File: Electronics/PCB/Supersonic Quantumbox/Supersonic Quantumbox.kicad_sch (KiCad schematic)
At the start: 41 parts, among them J1 USB_C_Receptacle_USB2.0, U1 Input_jack, U2 TL071, U3 PCM1808PWR, U4 AZ1117-5.0, U5 ESP32-S2-WROVER-I, U6 AZ1117-3.3, U7 PCM5100, U8 Output_jack

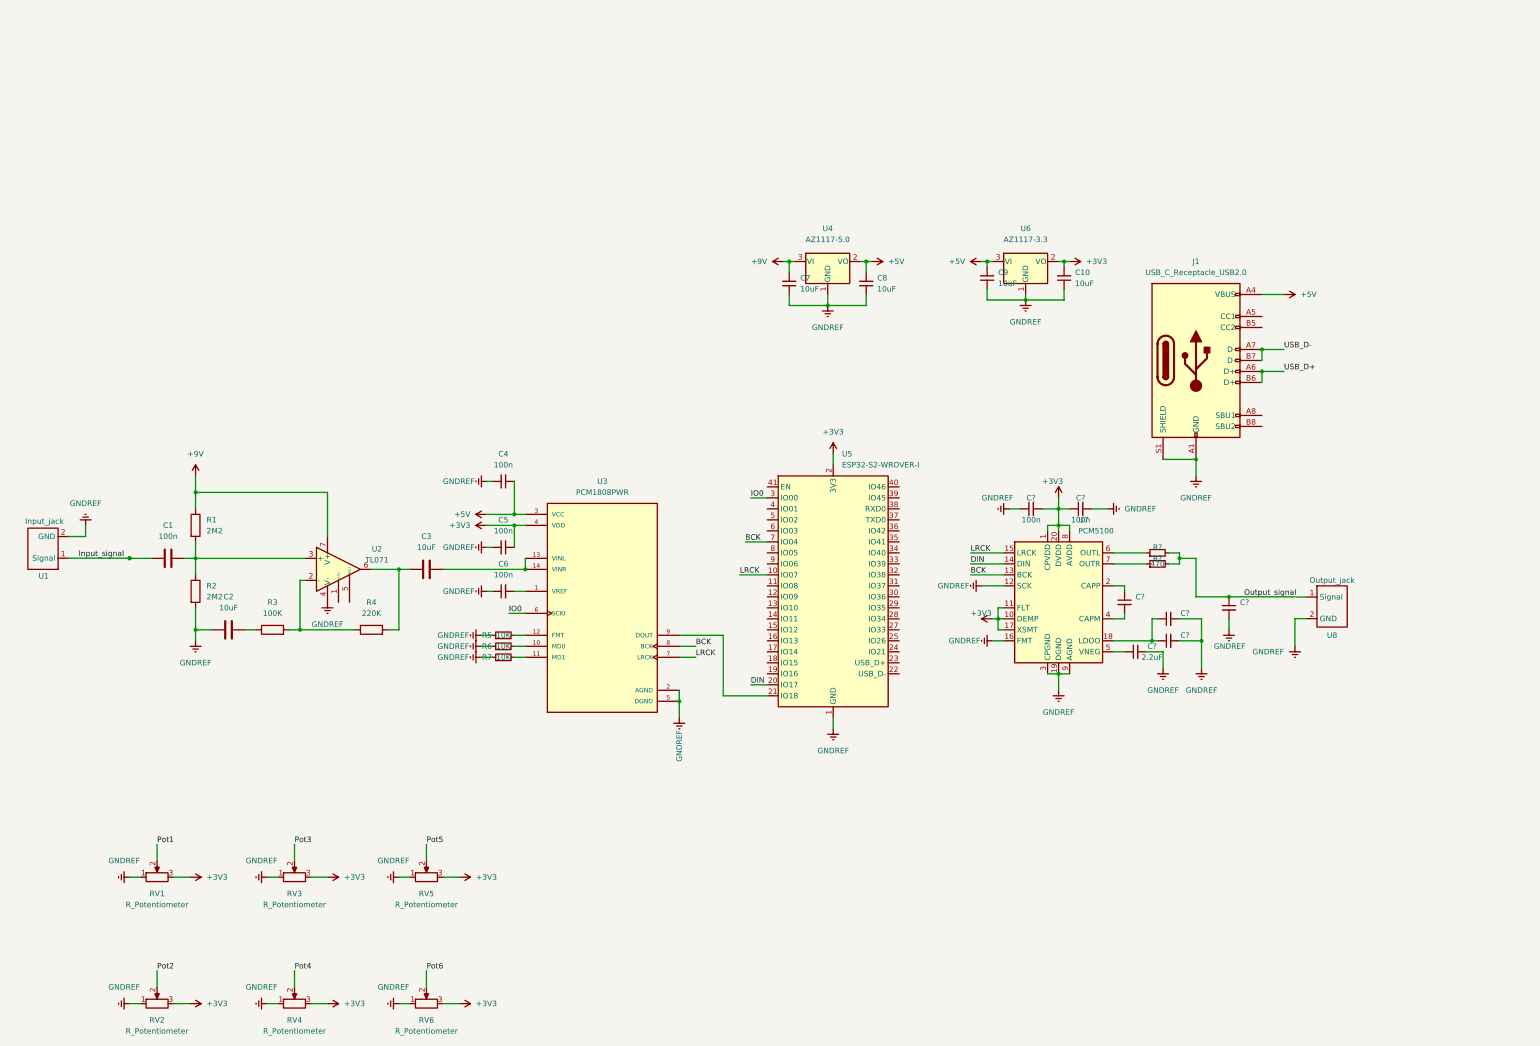
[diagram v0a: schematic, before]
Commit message: Start work on PCB
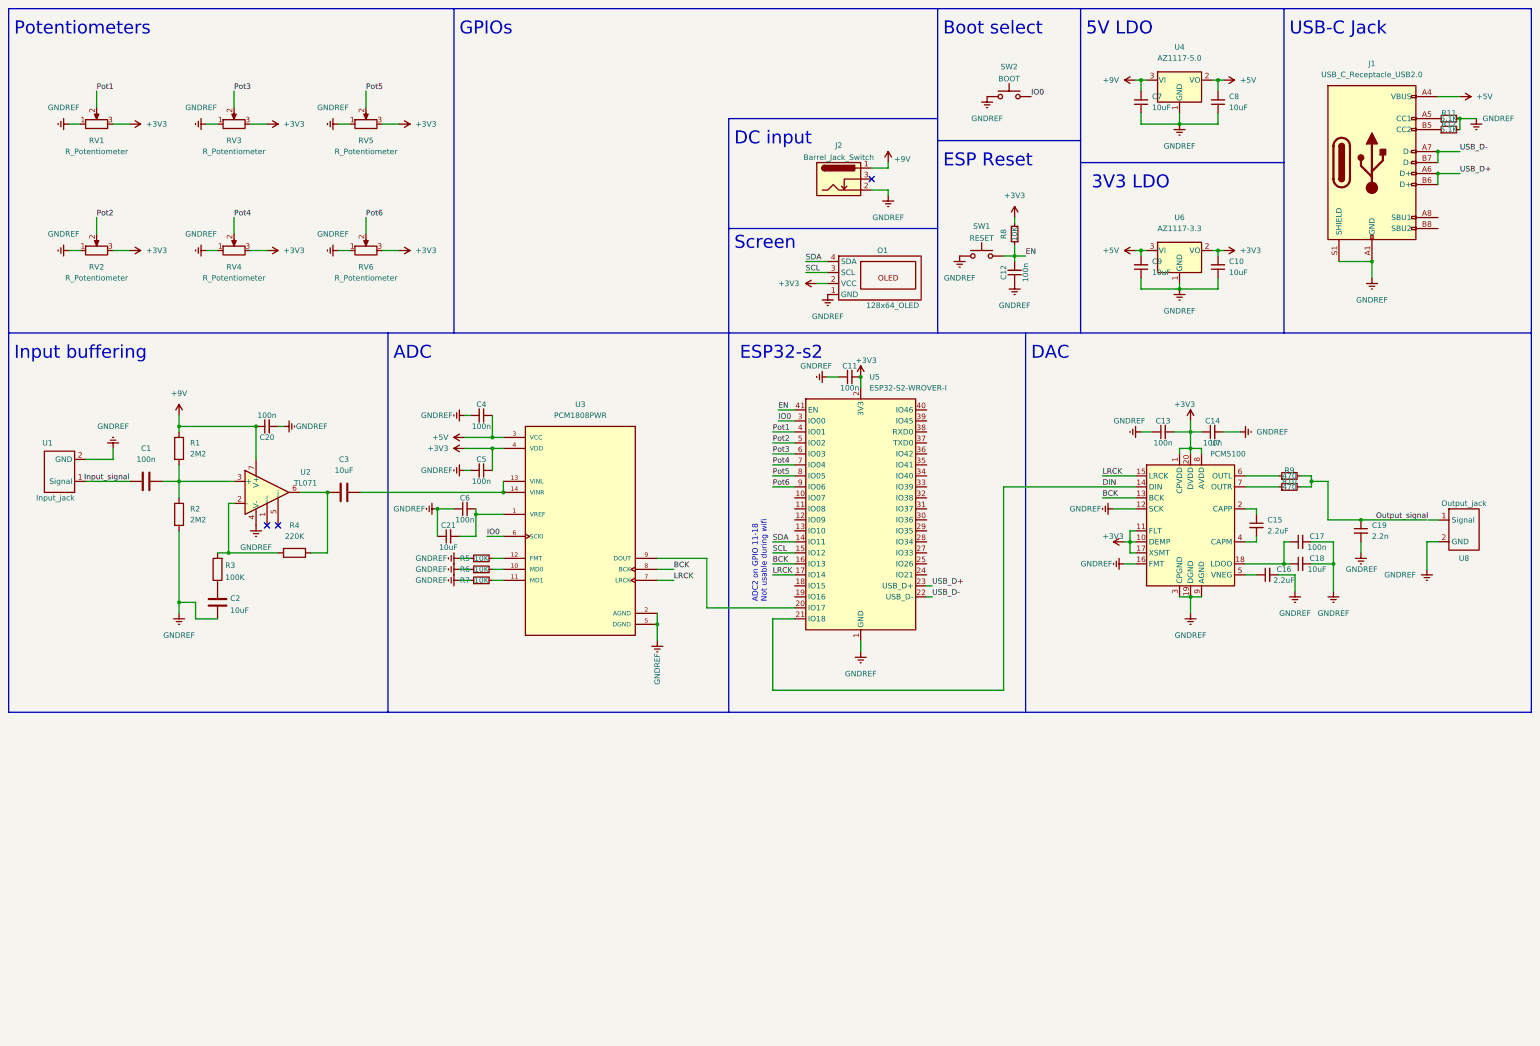
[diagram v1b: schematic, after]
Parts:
- added C11, C12, C20: 100n, Capacitor_SMD:C_0805_2012Metric_Pad1.18x1.45mm_HandSolder, symbol Device:C_Small
- added C21: 10uF, Capacitor_SMD:C_1206_3216Metric, symbol Device:C_Small
- added J2: Barrel_Jack_Switch, Connector_BarrelJack:BarrelJack_Horizontal, symbol Connector:Barrel_Jack_Switch
- added O1: 128x64_OLED, SupersonicQuantumbox:128x64OLED, symbol SupersonicQuantumbox:128x64_OLED
- added R11, R12: 5.1K, Resistor_SMD:R_0805_2012Metric_Pad1.20x1.40mm_HandSolder, symbol Device:R_Small
- added R8: 10K, Resistor_SMD:R_0805_2012Metric_Pad1.20x1.40mm_HandSolder, symbol Device:R_Small
- added SW1: RESET, Button_Switch_SMD:SW_Push_1P1T_NO_6x6mm_H9.5mm, symbol Switch:SW_Push
- added SW2: BOOT, Button_Switch_SMD:SW_Push_1P1T_NO_6x6mm_H9.5mm, symbol Switch:SW_Push
- C1, C4, C5, C6: footprint (none) -> Capacitor_SMD:C_0805_2012Metric_Pad1.18x1.45mm_HandSolder
- C10, C2, C3, C7, C8, C9: footprint (none) -> Capacitor_SMD:C_1206_3216Metric
- C13, C14: renamed from C?; footprint (none) -> Capacitor_SMD:C_0805_2012Metric_Pad1.18x1.45mm_HandSolder
- C15: renamed from C?; value (none) -> 2.2uF; footprint (none) -> Capacitor_SMD:C_1206_3216Metric
- C16: renamed from C?; footprint (none) -> Capacitor_SMD:C_1206_3216Metric
- C17: renamed from C?; value (none) -> 100n; footprint (none) -> Capacitor_SMD:C_0805_2012Metric_Pad1.18x1.45mm_HandSolder
- C18: renamed from C?; value (none) -> 10uF; footprint (none) -> Capacitor_SMD:C_1206_3216Metric
- C19: renamed from C?; value (none) -> 2.2n; footprint (none) -> Capacitor_SMD:C_0805_2012Metric_Pad1.18x1.45mm_HandSolder
- R1, R2, R3, R4, R5, R6, R7: footprint (none) -> Resistor_SMD:R_0805_2012Metric_Pad1.20x1.40mm_HandSolder
- R10: renamed from R?; footprint (none) -> Resistor_SMD:R_0805_2012Metric_Pad1.20x1.40mm_HandSolder
- R9: renamed from R?; value (none) -> 470; footprint (none) -> Resistor_SMD:R_0805_2012Metric_Pad1.20x1.40mm_HandSolder
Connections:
- net +3V3: now also C11.2, O1.2 (VCC), R8.2
- net +9V: now also C20.1, J2.1
- net BCK: now also U5.16 (IO13); no longer U5.7 (IO04)
- net DIN: now also U5.21 (IO18); no longer U5.20 (IO17)
- net GNDREF: now also C11.1, C12.1, C20.2, C21.1, J2.2, O1.1 (GND), R11.2, R12.2, SW1.1, SW2.1
- net IO0: now also SW2.2
- net LRCK: now also U5.17 (IO14); no longer U5.10 (IO07)
- net Pot1: now also U5.4 (IO01)
- net Pot2: now also U5.5 (IO02)
- net Pot3: now also U5.6 (IO03)
- net Pot4: now also U5.7 (IO04)
- net Pot5: now also U5.8 (IO05)
- net Pot6: now also U5.9 (IO06)
- net USB_D+: now also U5.23 (USB_D+)
- net USB_D-: now also U5.22 (USB_D-)
- net at C6.2, U3.1 (VREF): now also C21.2
- net at U3.9 (DOUT): now also U5.20 (IO17); no longer U5.21 (IO18)
- net SDA: now reaches U5.14 (IO11)
- net SDA: now also O1.4 (SDA)
- net SCL: now reaches U5.15 (IO12)
- net SCL: now also O1.3 (SCL)
- net EN: now reaches U5.41 (EN)
- net EN: now also C12.2, R8.1, SW1.2
- net at J1.A5 (CC1): now also R11.1
- net at J1.B5 (CC2): now also R12.1
- no-connect marks 0 -> 3
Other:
- note added: "3V3 LDO"
- note added: "5V LDO"
- note added: "ADC"
- note added: "ADC2 on GPIO 11-18 Not usable during wifi"
- note added: "Boot select"
- note added: "DAC"
- note added: "DC input"
- note added: "ESP Reset"
- note added: "ESP32-s2"
- note added: "GPIOs"
- note added: "Input buffering"
- note added: "Potentiometers"
- note added: "Screen"
- note added: "USB-C Jack"
- moved on the sheet: C1, C10, C13, C14, C15, C16, C17, C18, C19, C2, C3, C4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
